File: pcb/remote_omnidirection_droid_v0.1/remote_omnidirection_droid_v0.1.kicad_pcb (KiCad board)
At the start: 2 copper layers, 120 x 103.9 mm, 36 parts, among them J1 USB_C_Receptacle_USB2.0, J4 Conn_01x02, Q1 BC846BS, SW1 SW_SPST, U1 USBLC6-2SC6, U3 AZ1117-3.3, U4 AZ1117-5.0, U5 ESP32-S3-WROOM-2-N32R8V

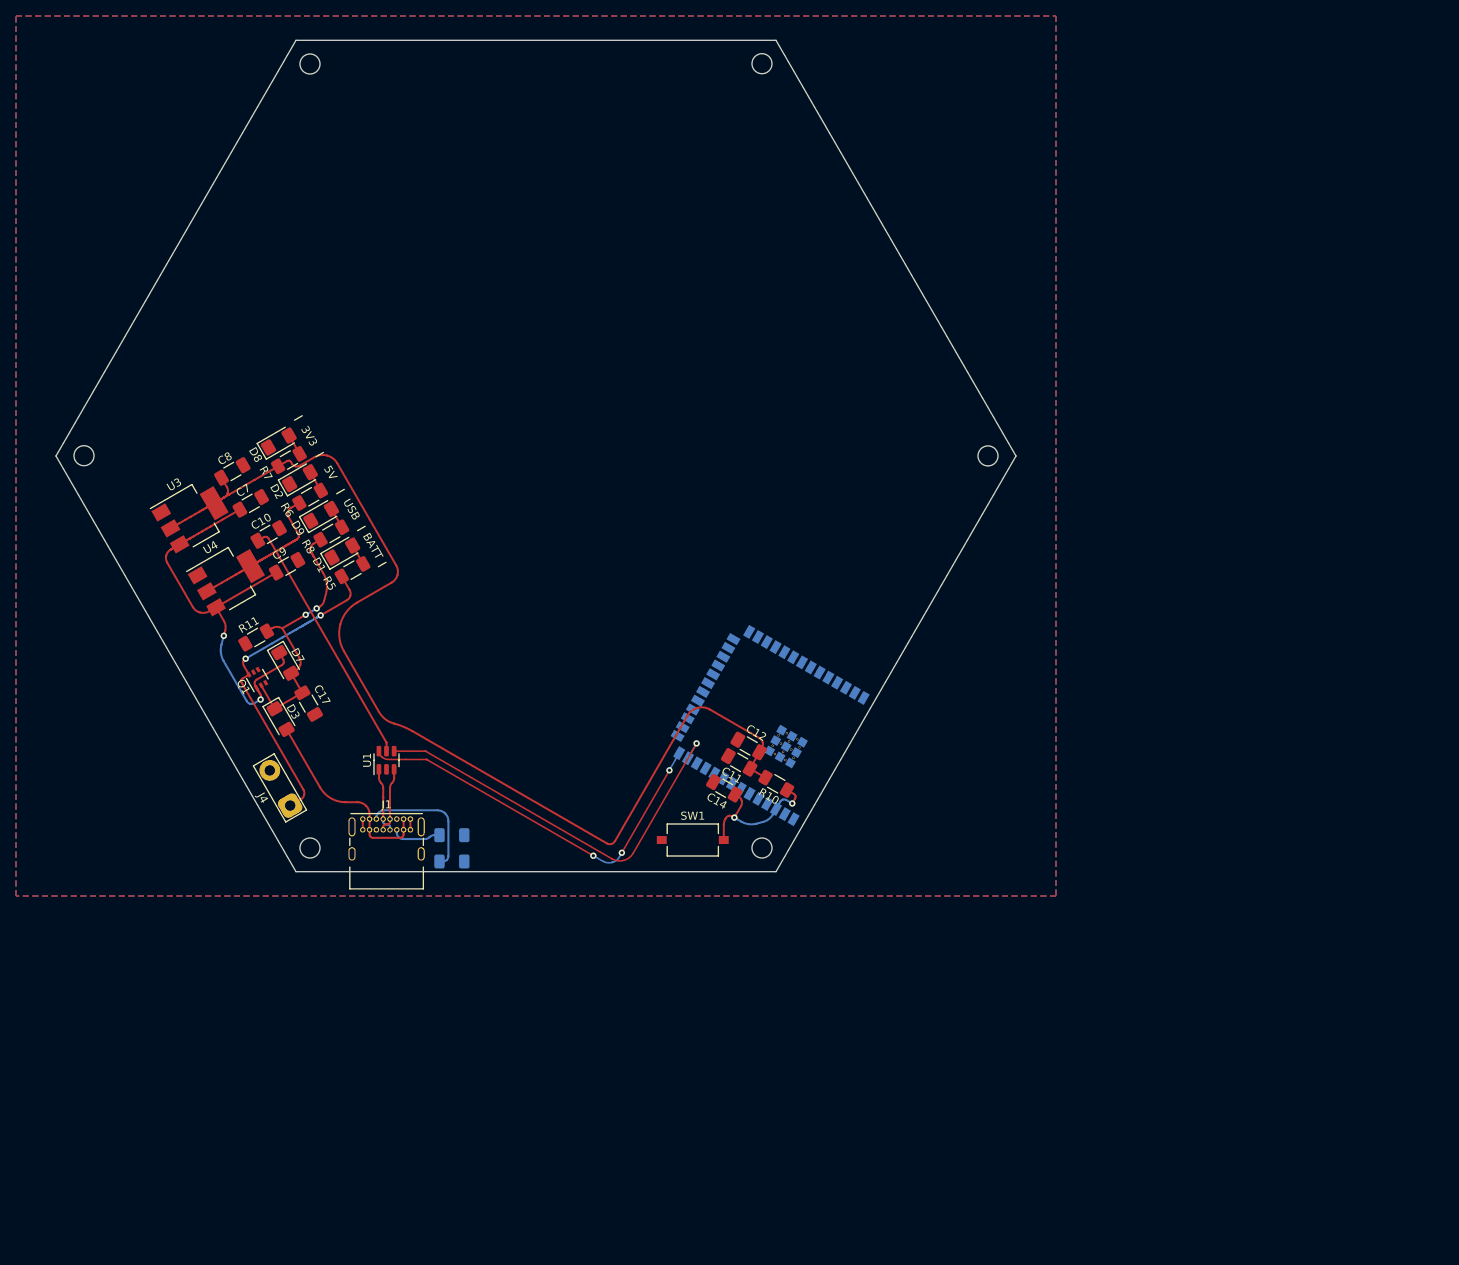
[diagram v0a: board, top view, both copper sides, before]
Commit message: updated PCB
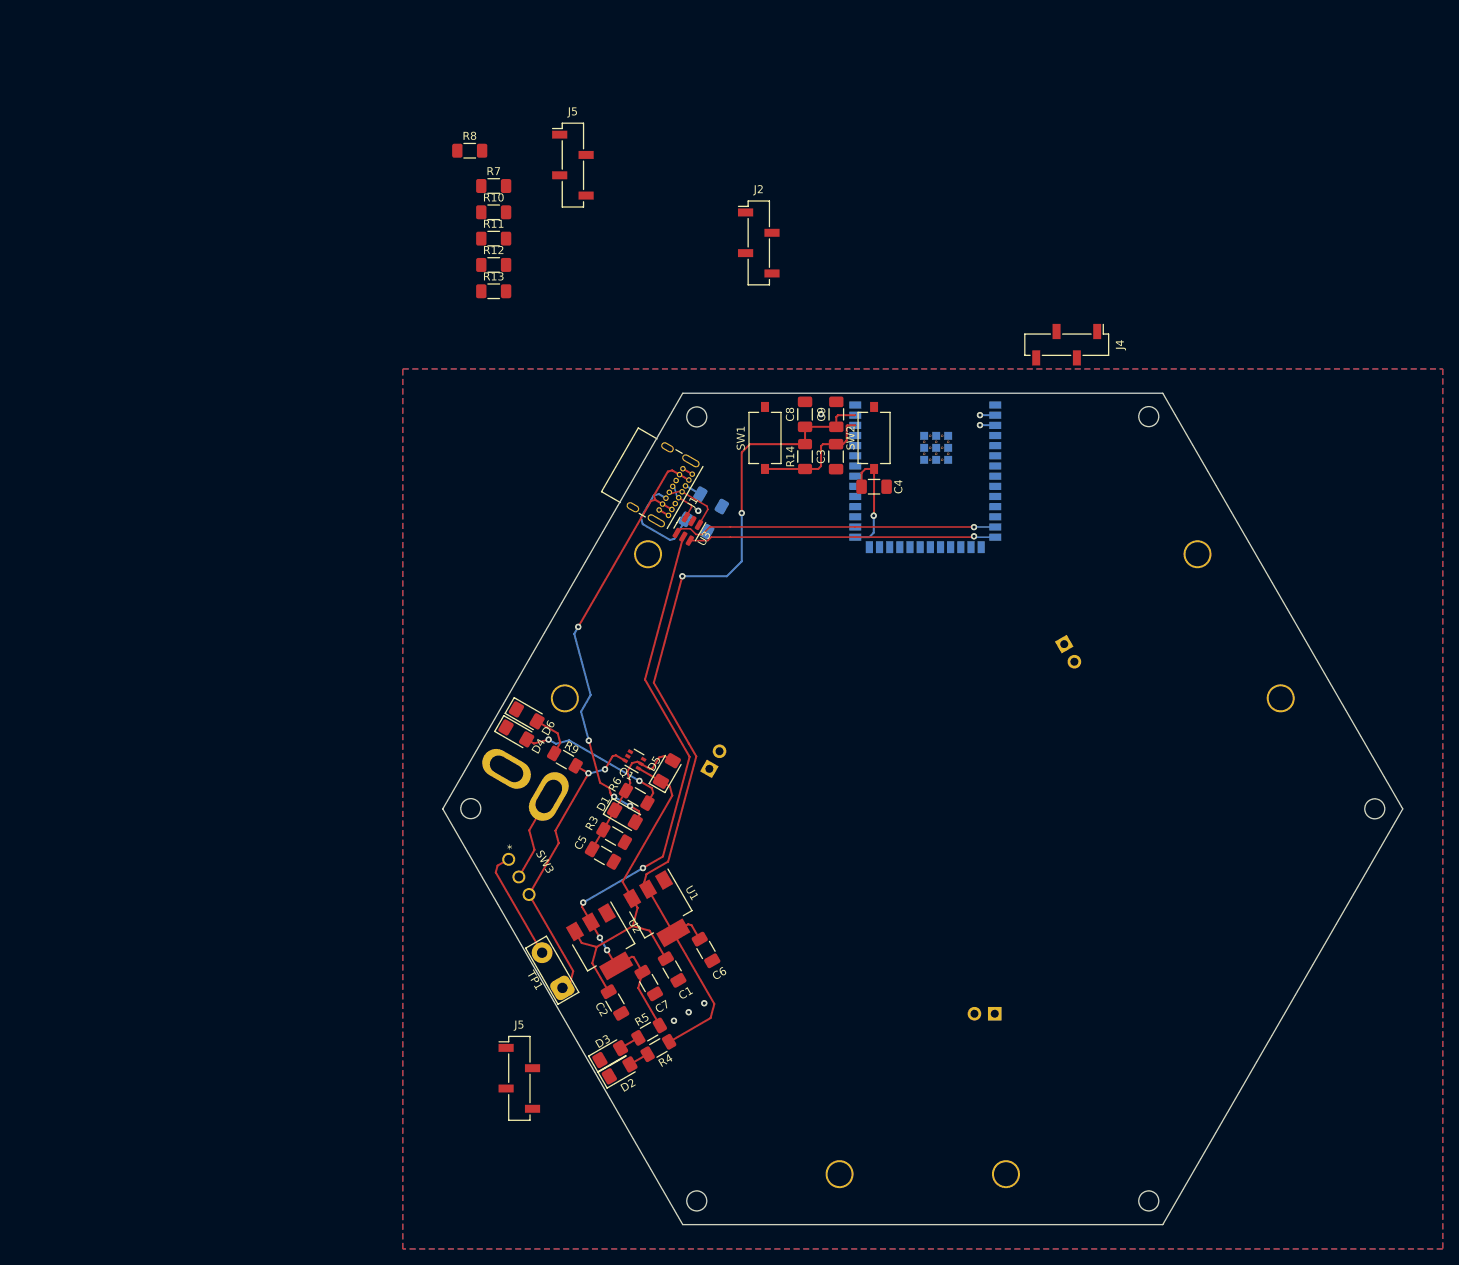
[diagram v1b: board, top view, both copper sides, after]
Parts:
- removed C10, C11: 22u, Capacitor_SMD:C_1206_3216Metric_Pad1.33x1.80mm_HandSolder
- removed C12, C14: 0.1u, Capacitor_SMD:C_1206_3216Metric_Pad1.33x1.80mm_HandSolder
- removed C17: 10u, Capacitor_SMD:C_1206_3216Metric_Pad1.33x1.80mm_HandSolder
- removed D7: MSK4005, Diode_SMD:D_1206_3216Metric_Pad1.42x1.75mm_HandSolder
- removed D8, D9: LED, LED_SMD:LED_1206_3216Metric_Pad1.42x1.75mm_HandSolder
- removed U5: ESP32-S3-WROOM-2-N32R8V, ESP32 S3:XCVR_ESP32-S3-WROOM-2-N32R8V
- added C1: 22u, Capacitor_SMD:C_1206_3216Metric_Pad1.33x1.80mm_HandSolder, F.Cu at (114.8, 153.0)
- added C2: 22u, Capacitor_SMD:C_1206_3216Metric_Pad1.33x1.80mm_HandSolder, F.Cu at (107.6, 157.1)
- added C3: 0.1u, Capacitor_SMD:C_1206_3216Metric_Pad1.33x1.80mm_HandSolder, F.Cu at (135.3, 88.9)
- added C4: 0.1u, Capacitor_SMD:C_1206_3216Metric_Pad1.33x1.80mm_HandSolder, F.Cu at (140.0, 92.6)
- added C5: 10u, Capacitor_SMD:C_1206_3216Metric_Pad1.33x1.80mm_HandSolder, F.Cu at (106.1, 138.7)
- added C6: 22u, Capacitor_SMD:C_1206_3216Metric_Pad1.33x1.80mm_HandSolder, F.Cu at (119.0, 150.5)
- added D4: LED, LED_SMD:LED_1206_3216Metric_Pad1.42x1.75mm_HandSolder, F.Cu at (95.3, 123.5)
- added D5: MSK4005, Diode_SMD:D_1206_3216Metric_Pad1.42x1.75mm_HandSolder, F.Cu at (114.1, 128.2)
- added D6: LED, LED_SMD:LED_1206_3216Metric_Pad1.42x1.75mm_HandSolder, F.Cu at (96.6, 121.2)
- added J2: Conn_01x04, Connector_PinSocket_2.54mm:PinSocket_1x04_P2.54mm_Vertical_SMD_Pin1Left, F.Cu at (125.6, 62.2)
- added J3: BATT_CONNECT, myparts:Deans T-Plug Header, B.Cu at (96.5, 129.7)
- added J5: Conn_01x04, Connector_PinSocket_2.54mm:PinSocket_1x04_P2.54mm_Vertical_SMD_Pin1Left, F.Cu at (102.4, 52.4)
- added J5: Conn_01x04, Connector_PinSocket_2.54mm:PinSocket_1x04_P2.54mm_Vertical_SMD_Pin1Left, F.Cu at (95.7, 166.6)
- added M1: Motor_DC_ALT, pimoroni_motor_breakout:Pimoroni_Motor_Breakout, B.Cu at (115.6, 115.3)
- added M2: Motor_DC_ALT, pimoroni_motor_breakout:Pimoroni_Motor_Breakout, B.Cu at (176.6, 115.3)
- added M3: Motor_DC_ALT, pimoroni_motor_breakout:Pimoroni_Motor_Breakout, B.Cu at (146.1, 168.1)
- added R12: 10k, Resistor_SMD:R_1206_3216Metric_Pad1.30x1.75mm_HandSolder, F.Cu at (92.5, 64.9)
- added R13: 10k, Resistor_SMD:R_1206_3216Metric_Pad1.30x1.75mm_HandSolder, F.Cu at (92.5, 68.2)
- added R14: 10k, Resistor_SMD:R_1206_3216Metric_Pad1.30x1.75mm_HandSolder, F.Cu at (131.4, 88.9)
- added R3: 100k, Resistor_SMD:R_1206_3216Metric_Pad1.30x1.75mm_HandSolder, F.Cu at (107.5, 136.3)
- added R4: 220, Resistor_SMD:R_1206_3216Metric_Pad1.30x1.75mm_HandSolder, F.Cu at (113.1, 162.8)
- added R9: 220, Resistor_SMD:R_1206_3216Metric_Pad1.30x1.75mm_HandSolder, F.Cu at (101.4, 126.7)
- added SW2: SW_SPST, Button_Switch_SMD:SW_Tactile_SPST_NO_Straight_CK_PTS636Sx25SMTRLFS, F.Cu at (140.0, 86.5)
- added SW3: SW_SPDT, myparts:SWITCH_25336NA_APM, F.Cu at (94.4, 139.2)
- added TP1: AMMETER_CONN, TestPoint:TestPoint_2Pads_Pitch5.08mm_Drill1.3mm, F.Cu at (101.1, 155.3)
- added U2: AZ1117-5.0, Package_TO_SOT_SMD:SOT-223-3_TabPin2, F.Cu at (106.2, 149.8)
- C8: value 22u -> 0.1u
- D1: value LED -> MSK4005; footprint LED_SMD:LED_1206_3216Metric_Pad1.42x1.75mm_HandSolder -> Diode_SMD:D_1206_3216Metric_Pad1.42x1.75mm_HandSolder
- D3: value MSK4005 -> LED; footprint Diode_SMD:D_1206_3216Metric_Pad1.42x1.75mm_HandSolder -> LED_SMD:LED_1206_3216Metric_Pad1.42x1.75mm_HandSolder
- J4: value Conn_01x02 -> Conn_01x04; footprint TestPoint:TestPoint_2Pads_Pitch5.08mm_Drill1.3mm -> Connector_PinSocket_2.54mm:PinSocket_1x04_P2.54mm_Vertical_SMD_Pin1Left
- R11: value 100k -> 10k
- R7, R8: value 220 -> 10k
- U1: value USBLC6-2SC6 -> AZ1117-3.3; footprint Package_TO_SOT_SMD:SOT-23-6 -> Package_TO_SOT_SMD:SOT-223-3_TabPin2
- U3: value AZ1117-3.3 -> USBLC6-2SC6; footprint Package_TO_SOT_SMD:SOT-223-3_TabPin2 -> Package_TO_SOT_SMD:SOT-23-6
- U4: value AZ1117-5.0 -> ESP32-S3-WROOM-2-N32R8V; footprint Package_TO_SOT_SMD:SOT-223-3_TabPin2 -> ESP32 S3:XCVR_ESP32-S3-WROOM-2-N32R8V; moved to B.Cu
- moved J4 112.9 mm to (164.1, 74.9), turned to -90 degrees
- moved U4 88.6 mm to (146.4, 87.7), turned to 180 degrees
- moved D2 84.1 mm to (108.2, 165.6)
- moved R10 79.7 mm to (92.5, 58.3), turned to 0 degrees
- moved C7 77.9 mm to (111.9, 154.7), turned to -60 degrees
- moved C8 71.9 mm to (131.4, 83.6), turned to 90 degrees
- moved C9 71.2 mm to (135.3, 83.6), turned to 90 degrees
- moved R5 68.6 mm to (111.9, 160.7), turned to -150 degrees
- moved H6 65.4 mm to (117.9, 181.9)
- moved H3 65.4 mm to (174.4, 83.9)
- moved H2 65.4 mm to (117.9, 83.9)
- moved H5 65.4 mm to (174.4, 181.9)
- moved H4 65.4 mm to (202.6, 132.9)
- moved H1 65.4 mm to (89.6, 132.9)
- moved U3 62.0 mm to (116.7, 97.9), turned to -120 degrees
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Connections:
- net Net-(J1-CC1) renamed /CC1
- net Net-(J1-CC2) renamed /CC2
- C7 pad 1: VCC -> +5V
- C9 pad 1: VCC -> +3V3
- D1 pad 1: GND -> Net-(D1-K)
- D1 pad 2: Net-(D1-A) -> VBUS
- D3 pad 1: /LED_USB -> GND
- D3 pad 2: VBUS -> Net-(D3-A)
- J1 pad A6: Net-(J1-D+-PadA6) -> /NESD_D+
- J1 pad A7: Net-(J1-D--PadA7) -> /NESD_D-
- J1 pad B6: Net-(J1-D+-PadA6) -> /NESD_D+
- J1 pad B7: Net-(J1-D--PadA7) -> /NESD_D-
- J4 pad 1: +BATT -> +5V
- J4 pad 2: GND -> /TRIG2
- Q1 pad 2: /LED_USB -> Net-(D1-K)
- R10 pad 1: /EN -> /ECHO2
- R10 pad 2: +3V3 -> Net-(J4-Pin_3)
- R11 pad 1: GND -> Net-(J4-Pin_3)
- R11 pad 2: /LED_USB -> GND
- R5 pad 1: +BATT -> +5V
- R5 pad 2: Net-(D1-A) -> Net-(D3-A)
- R6 pad 1: +5V -> Net-(D1-K)
- R6 pad 2: Net-(D2-A) -> Net-(D4-A)
- R7 pad 1: +3V3 -> /ECHO1
- R7 pad 2: Net-(D8-A) -> Net-(J2-Pin_3)
- R8 pad 1: /LED_USB -> Net-(J2-Pin_3)
- R8 pad 2: Net-(D9-A) -> GND
- U1 pad 1: Net-(J1-D+-PadA6) -> GND
- U1 pad 2: GND -> +3V3
- U1 pad 3: Net-(J1-D--PadA7) -> VCC
- U3 pad 1: GND -> /NESD_D+
- U3 pad 2: +3V3 -> GND
- U3 pad 3: VCC -> /NESD_D-
- U4 pad 2: +5V -> +3V3
- U4 pad 3: VCC -> /EN
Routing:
- net /LED_USB: track 33.5 -> 0.00 mm, vias 2 -> 0
- net VBUS: track 25.2 -> 56.4 mm, vias 0 -> 4
- net +5V: track 52.8 -> 75.2 mm, vias 0 -> 4
- net +3V3: track 134.5 -> 114.0 mm, vias 0 -> 3
- net Net-(D4-A): track 0.00 -> 19.8 mm, vias 0 -> 2
- net Net-(D1-K): track 0.00 -> 18.6 mm
- net /CC1: track 16.3 -> 2.14 mm
- net Net-(SW3-A): track 0.00 -> 14.1 mm
- net /BOOT: track 0.00 -> 14.0 mm, vias 0 -> 1
- net Net-(J3-Pin_1): track 0.00 -> 11.3 mm
- net /D-: track 51.9 -> 40.7 mm
- net /D+: track 49.3 -> 38.4 mm, vias 3 -> 1
- net Net-(J1-D+-PadA6): track 8.28 -> 0.00 mm
- net Net-(J1-D--PadA7): track 8.28 -> 0.00 mm
- net /NESD_D+: track 0.00 -> 7.94 mm
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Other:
- board text removed: "3V3"
- board text removed: "5V"
- board text removed: "BATT"
- board text removed: "USB"
